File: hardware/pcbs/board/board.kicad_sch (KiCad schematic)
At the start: 66 parts, among them K00 Key, K01 Key, K02 Key, K03 Key, K10 Key, K11 Key, K12 Key, K13 Key, K20 Key, K21 Key, K22 Key, K23 Key, K30 Key, K31 Key, K32 Key, K33 Key, K40 Key, K41 Key, K42 Key, K43 Key, K50 Key, K51 Key, K52 Key, K53 Key, K60 Key, K61 Key

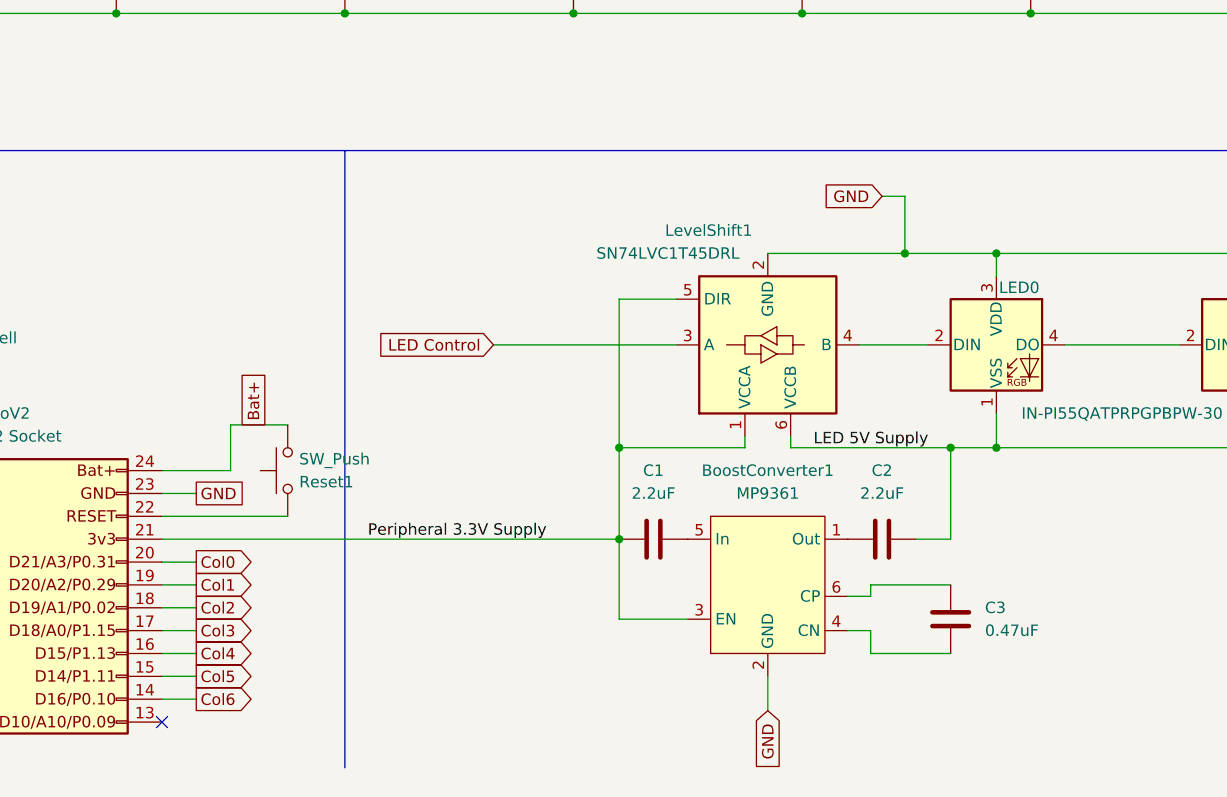
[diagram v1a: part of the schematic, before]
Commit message: pcb updates
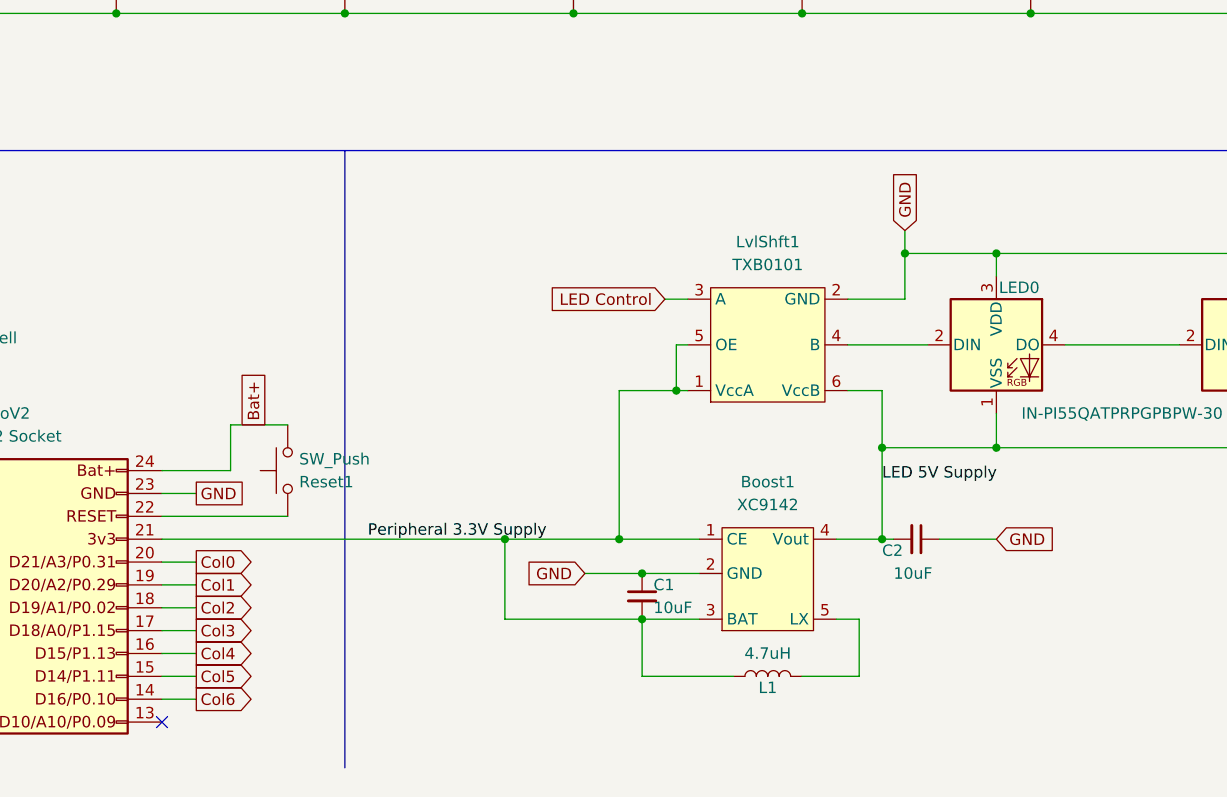
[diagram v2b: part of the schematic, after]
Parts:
- removed BoostConverter1: MP9361, Package_TO_SOT_SMD:SOT-23-6, symbol SVastaCustomParts:MP9361
- removed C1, C2: 2.2uF, Capacitor_SMD:C_0805_2012Metric_Pad1.18x1.45mm_HandSolder, symbol Device:C
- removed C3: 0.47uF, Capacitor_SMD:C_0805_2012Metric_Pad1.18x1.45mm_HandSolder, symbol Device:C
- removed LevelShift1: SN74LVC1T45DRL, Package_TO_SOT_SMD:SOT-563, symbol Logic_LevelTranslator:SN74LVC1T45DRL
- added Boost1: XC9142, SVastaCustomParts:SOT-25-5, symbol SVastaCustomParts:XC9142
- added C1, C2: 10uF, Capacitor_SMD:C_0805_2012Metric_Pad1.18x1.45mm_HandSolder, symbol Device:C_Small
- added L1: 4.7uH, Inductor_SMD:L_0805_2012Metric_Pad1.15x1.40mm_HandSolder, symbol Device:L
- added LvlShft1: TXB0101, Package_TO_SOT_SMD:SOT-23-6_Handsoldering, symbol SVastaCustomParts:TXB0101
- Battery1: footprint SVastaCustomParts:Battery Holder THT AA 1 Cell Keystone 1087 -> SVastaCustomParts:BatteryHolder_Keystone_1088_1xAA
- Nice!NanoV2: footprint Package_DIP:DIP-24_W15.24mm_Socket -> SVastaCustomParts:Nice!NanoSocket_Reversible
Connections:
- net GND: now also Boost1.2 (GND), C1.1, C2.1, LvlShft1.2 (GND)
- net LED 5V Supply: now also Boost1.4 (Vout), C2.2, LvlShft1.6 (VccB)
- net LED Control: now also LvlShft1.3 (A)
- net Peripheral 3.3V Supply: now also Boost1.1 (CE), Boost1.3 (BAT), C1.2, L1.1, LvlShft1.1 (VccA), LvlShft1.5 (OE)
- net at LED0.2 (DIN): now also LvlShft1.4 (B)
- new net: Boost1.5 (LX), L1.2

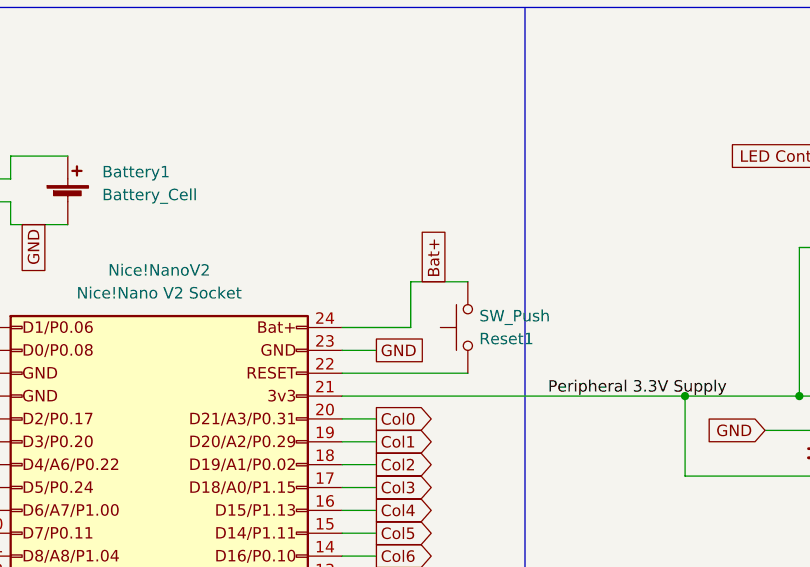
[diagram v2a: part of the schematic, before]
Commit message: stale updates from v1
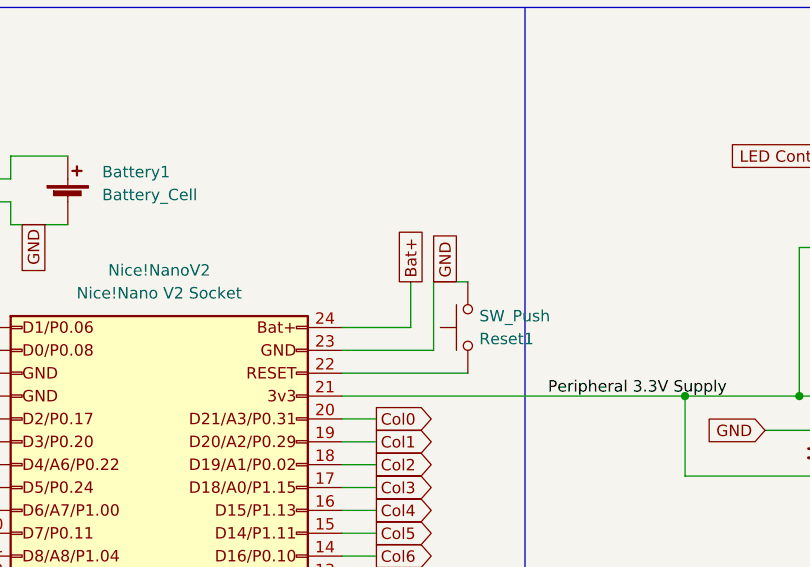
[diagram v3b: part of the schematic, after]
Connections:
- net Bat+: no longer Reset1.2
- net GND: now also Reset1.2
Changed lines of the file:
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@@
+    (stroke (width 0) (type default) (color 0 0 0 0))
+  )
+  (wire (pts (xy 82.55 167.64) (xy 82.55 160.02))
     (stroke (width 0) (type default) (color 0 0 0 0))
   )
@@
     (stroke (width 0) (type default) (color 0 0 0 0))
   )
-  (wire (pts (xy 72.39 167.64) (xy 76.2 167.64))
+  (wire (pts (xy 72.39 167.64) (xy 82.55 167.64))
     (stroke (width 0) (type default) (color 0 0 0 0))
   )
@@
     (stroke (width 0) (type default) (color 0 0 0 0))
   )
+  (wire (pts (xy 82.55 160.02) (xy 86.36 160.02))
+    (stroke (width 0) (type default) (color 0 0 0 0))
+  )
   (wire (pts (xy 50.8 30.48) (xy 57.15 30.48))
     (stroke (width 0) (type default) (color 0 0 0 0))
@@
   )
   (wire (pts (xy 118.11 88.9) (xy 143.51 88.9))
-    (stroke (width 0) (type default) (color 0 0 0 0))
-  )
-  (wire (pts (xy 80.01 160.02) (xy 86.36 160.02))
     (stroke (width 0) (type default) (color 0 0 0 0))
   )
@@
     )
   )
-  (global_label "Bat+" (shape passive) (at 82.55 160.02 90) (fields_autoplaced)
-    (effects (font (size 1.27 1.27)) (justify left))
-    (property "Intersheet References" "${INTERSHEET_REFS}" (id 0) (at 82.4706 152.8898 90)
+  (global_label "Bat+" (shape passive) (at 80.01 160.02 90) (fields_autoplaced)
+    (effects (font (size 1.27 1.27)) (justify left))
+    (property "Intersheet References" "${INTERSHEET_REFS}" (id 0) (at 79.9306 152.8898 90)
       (effects (font (size 1.27 1.27)) (justify left) hide)
     )
@@
     )
   )
-  (global_label "GND" (shape passive) (at 76.2 167.64 0) (fields_autoplaced)
-    (effects (font (size 1.27 1.27)) (justify left))
-    (property "Intersheet References" "${INTERSHEET_REFS}" (id 0) (at 82.4836 167.5606 0)
-      (effects (font (size 1.27 1.27)) (justify left) hide)
-    )
+  (global_label "GND" (shape passive) (at 83.82 160.02 90) (fields_autoplaced)
+    (effects (font (size 1.27 1.27)) (justify left))
+    (property "Intersheet References" "${INTERSHEET_REFS}" (id 0) (at 83.7406 153.7364 90)
+      (effects (font (size 1.27 1.27)) (justify left) hide)
+    )
